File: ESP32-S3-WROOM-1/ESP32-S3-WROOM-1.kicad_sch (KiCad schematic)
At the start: 19 parts, among them J1 ESP32-S3-DEVKITC-1-J1, J2 ESP32-S3-DEVKITC-1-J2, J3 ESP-Prog-ProgramCOM-RECV, J4 USB2.0_C_v3, SW1 RS, SW2 BT, U1 ESP32-S3-WROOM-1, U2 AMS1117-3.3

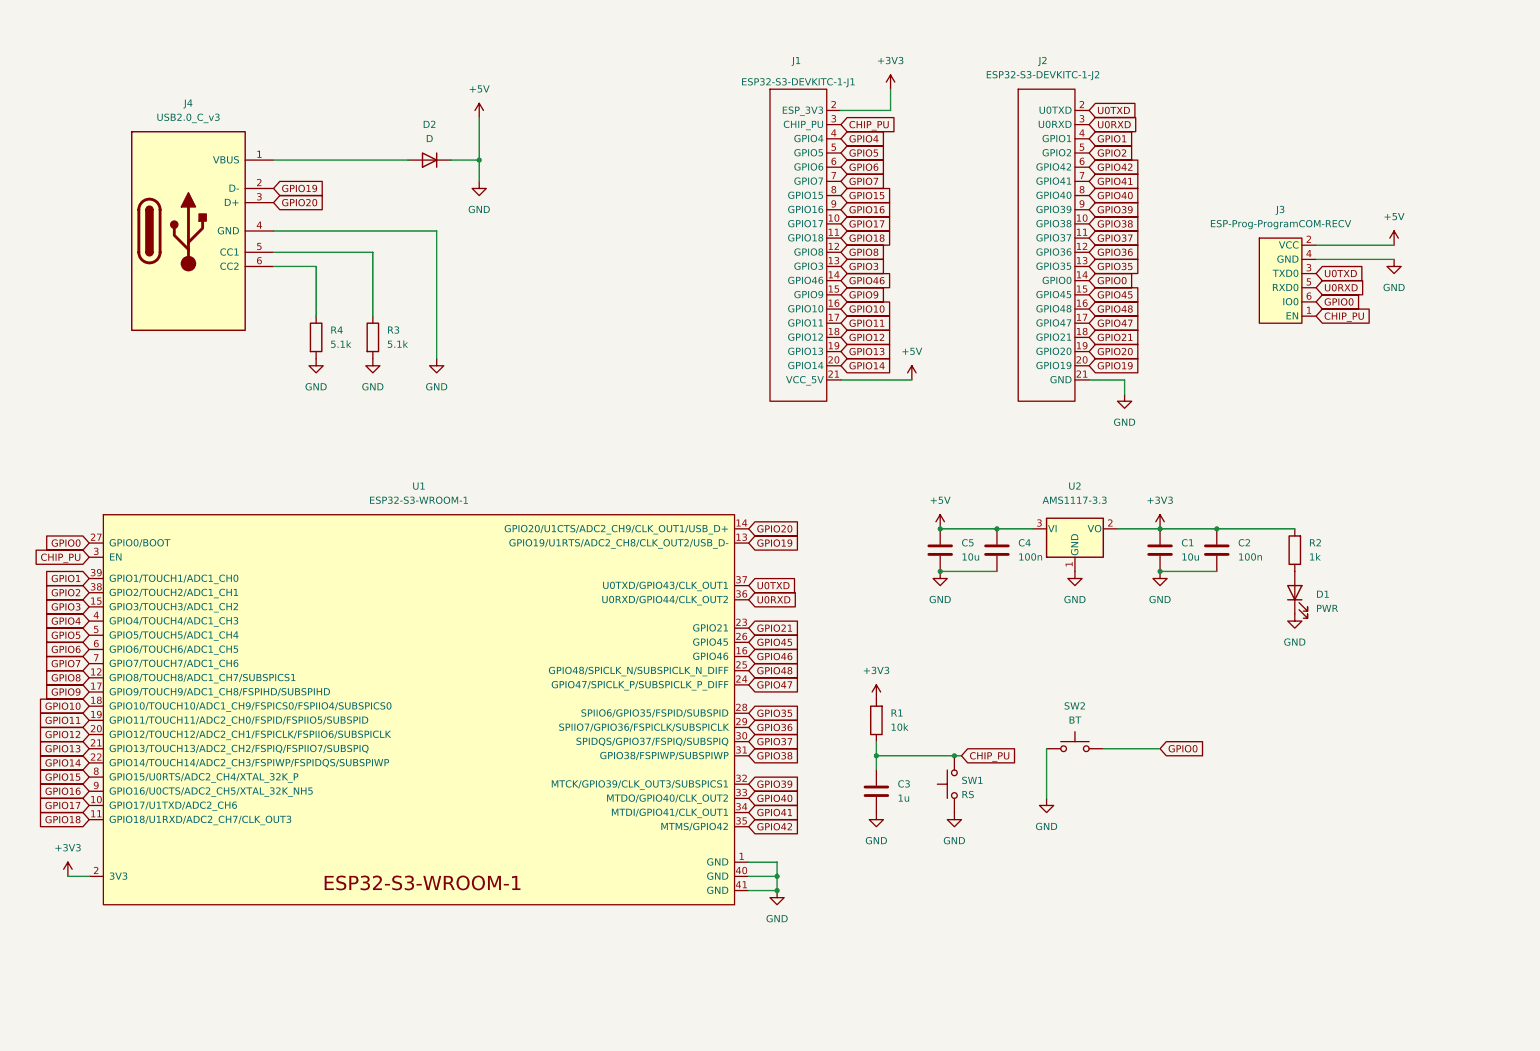
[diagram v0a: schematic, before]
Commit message: add title
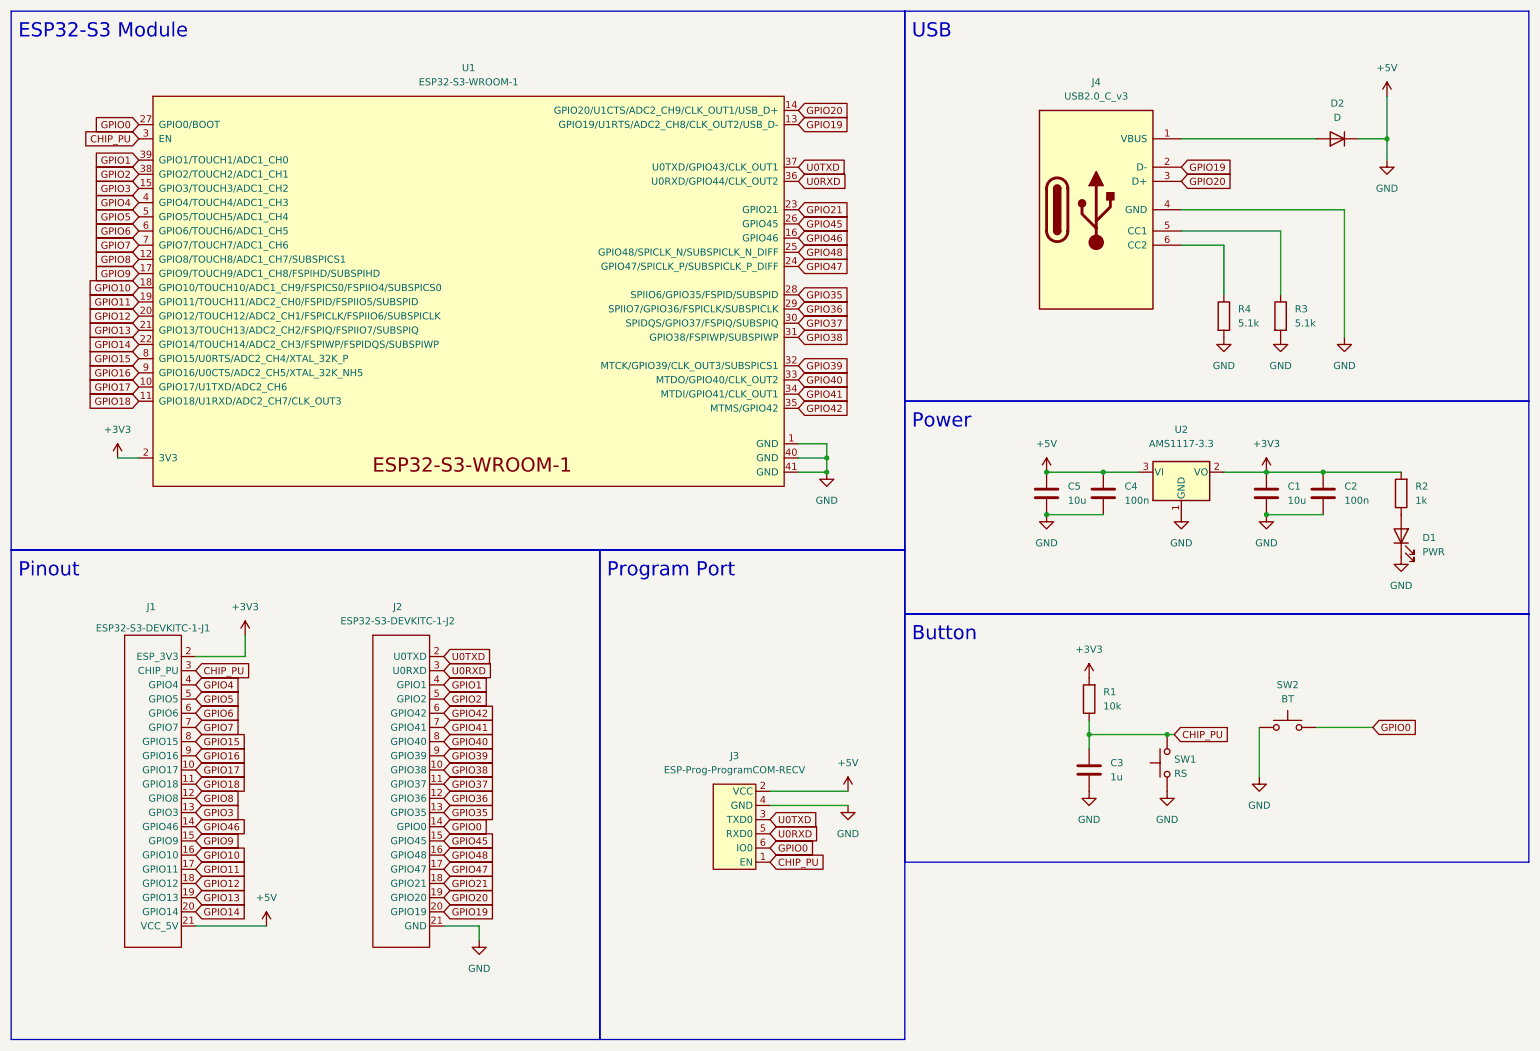
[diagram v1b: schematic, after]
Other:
- note added: "Button"
- note added: "ESP32-S3 Module"
- note added: "Pinout"
- note added: "Power"
- note added: "Program Port"
- note added: "USB"
- title: (none) -> ESP32-S3 Dev Board
- moved on the sheet: C1, C2, C3, C4, C5, D1, D2, J1, J2, J3, J4, R1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
